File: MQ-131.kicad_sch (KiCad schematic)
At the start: 11 parts, among them J1 Conn_01x04_Pin

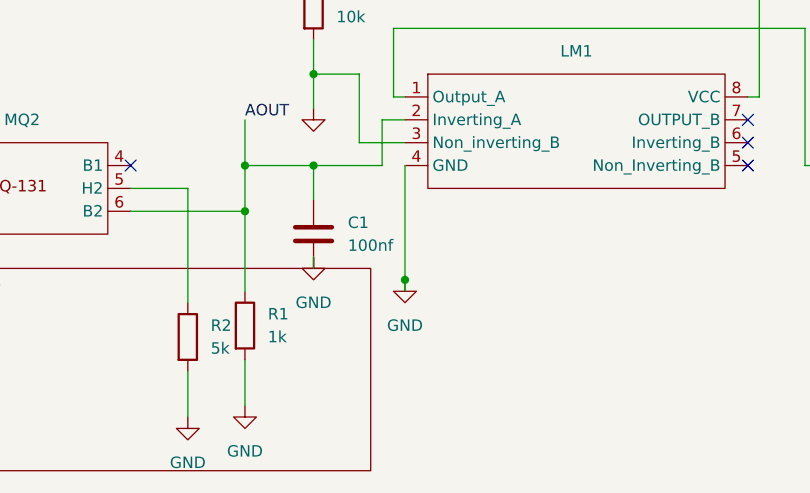
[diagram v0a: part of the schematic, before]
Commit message: PCB board design altered
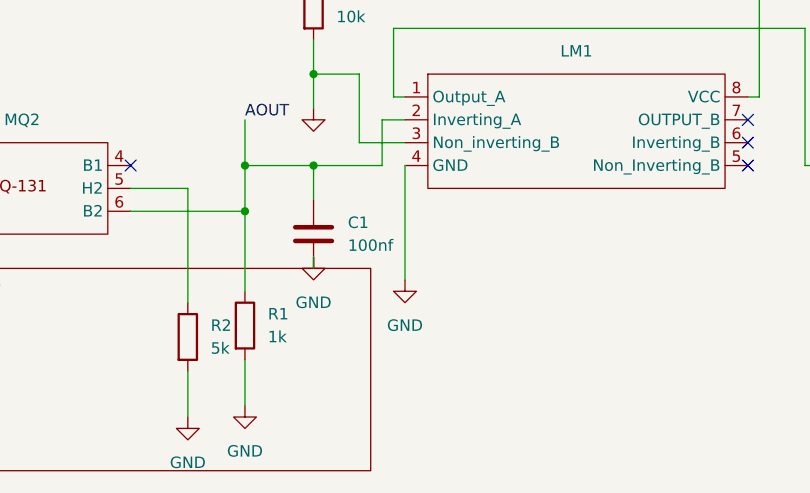
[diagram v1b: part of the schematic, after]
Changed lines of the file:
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@@
-	)
-	(junction
-		(at 166.37 85.09)
-		(diameter 0)
-		(color 0 0 0 0)
 	)
 	(junction
@@
 		(pts
 			(xy 156.21 46.99) (xy 156.21 50.8)
-		)
-		(stroke
-			(width 0)
-			(type default)
-		)
-	)
-	(wire
-		(pts
-			(xy 166.37 86.36) (xy 166.37 85.09)
 		)
 		(stroke
@@
 	)
 	(symbol
+		(lib_id "power:GND")
+		(at 166.37 85.09 0)
+		(unit 1)
+		(body_style 1)
+		(exclude_from_sim no)
+		(in_bom yes)
+		(on_board yes)
+		(in_pos_files yes)
+		(dnp no)
+		(fields_autoplaced yes)
+		(property "Reference" "#PWR012"
+			(at 166.37 91.44 0)
+			(hide yes)
+			(show_name no)
+			(do_not_autoplace no)
+			(effects
+				(font
+					(size 1.27 1.27)
+				)
+			)
+		)
+		(property "Value" "GND"
+			(at 166.37 90.17 0)
+			(show_name no)
+			(do_not_autoplace no)
+			(effects
+				(font
+					(size 1.27 1.27)
+				)
+			)
+		)
+		(property "Footprint" ""
+			(at 166.37 85.09 0)
+			(hide yes)
+			(show_name no)
+			(do_not_autoplace no)
+			(effects
+				(font
+					(size 1.27 1.27)
+				)
+			)
+		)
+		(property "Datasheet" ""
+			(at 166.37 85.09 0)
+			(hide yes)
+			(show_name no)
+			(do_not_autoplace no)
+			(effects
+				(font
+					(size 1.27 1.27)
+				)
+			)
+		)
+		(property "Description" "Power symbol creates a global label with name \"GND\" , ground"
+			(at 166.37 85.09 0)
+			(hide yes)
+			(show_name no)
+			(do_not_autoplace no)
+			(effects
+				(font
+					(size 1.27 1.27)
+				)
+			)
+		)
+		(pin "1"
+		)
+		(instances
+			(project "MQ-131"
+				(path "/9ab6dc58-de4d-4751-bedd-de9509a6e892"
+					(reference "#PWR012")
+					(unit 1)
+				)
+			)
+		)
+	)
+	(symbol
 		(lib_id "power:VCC")
 		(at 217.17 49.53 0)
@@
 					(unit 1)
 				)
-			)
-		)
-	)
-	(symbol
-		(lib_id "power:GND")
-		(at 166.37 85.09 0)
-		(unit 1)
-		(body_style 1)
-		(exclude_from_sim no)
-		(in_bom yes)
-		(on_board yes)
-		(in_pos_files yes)
-		(dnp no)
-		(fields_autoplaced yes)
-		(property "Reference" "#PWR012"
-			(at 166.37 91.44 0)
-			(hide yes)
-			(show_name no)
-			(do_not_autoplace no)
-			(effects
-				(font
-					(size 1.27 1.27)
-				)
-			)
-		)
-		(property "Value" "GND"
-			(at 166.37 90.17 0)
-			(show_name no)
-			(do_not_autoplace no)
-			(effects
-				(font
-					(size 1.27 1.27)
-				)
-			)
-		)
-		(property "Footprint" ""
-			(at 166.37 85.09 0)
-			(hide yes)
-			(show_name no)
-			(do_not_autoplace no)
-			(effects
-				(font
-					(size 1.27 1.27)
-				)
-			)
-		)
-		(property "Datasheet" ""
-			(at 166.37 85.09 0)
-			(hide yes)
-			(show_name no)
-			(do_not_autoplace no)
-			(effects
-				(font
-					(size 1.27 1.27)
-				)
-			)
-		)
-		(property "Description" "Power symbol creates a global label with name \"GND\" , ground"
-			(at 166.37 85.09 0)
-			(hide yes)
-			(show_name no)
-			(do_not_autoplace no)
-			(effects
-				(font
-					(size 1.27 1.27)
-				)
-			)
-		)
-		(pin "1"
-		)
-		(instances
-			(project "MQ-131"
-				(path "/9ab6dc58-de4d-4751-bedd-de9509a6e892"
-					(reference "#PWR012")
-					(unit 1)
-				)
